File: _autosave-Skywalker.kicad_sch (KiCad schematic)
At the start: 28 parts

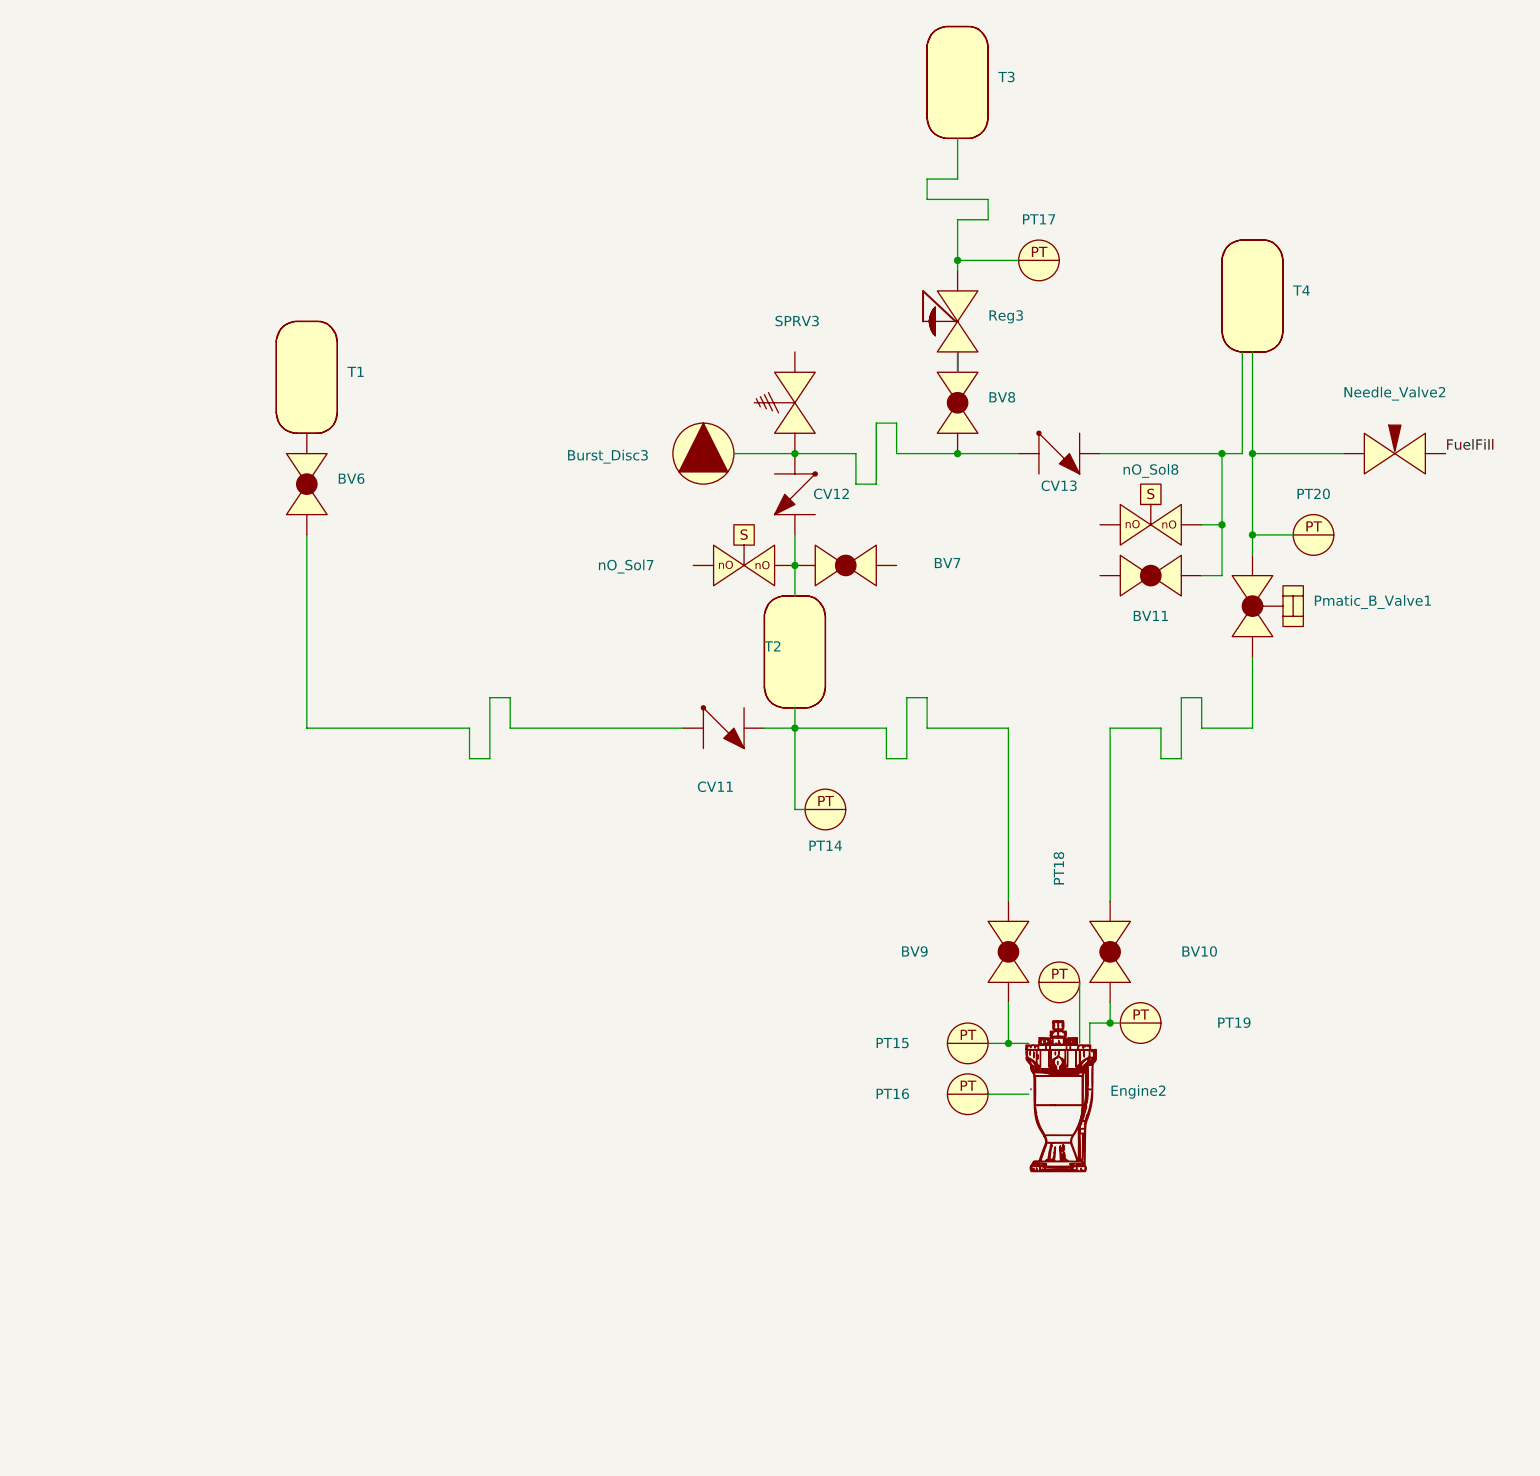
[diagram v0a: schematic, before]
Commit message: update
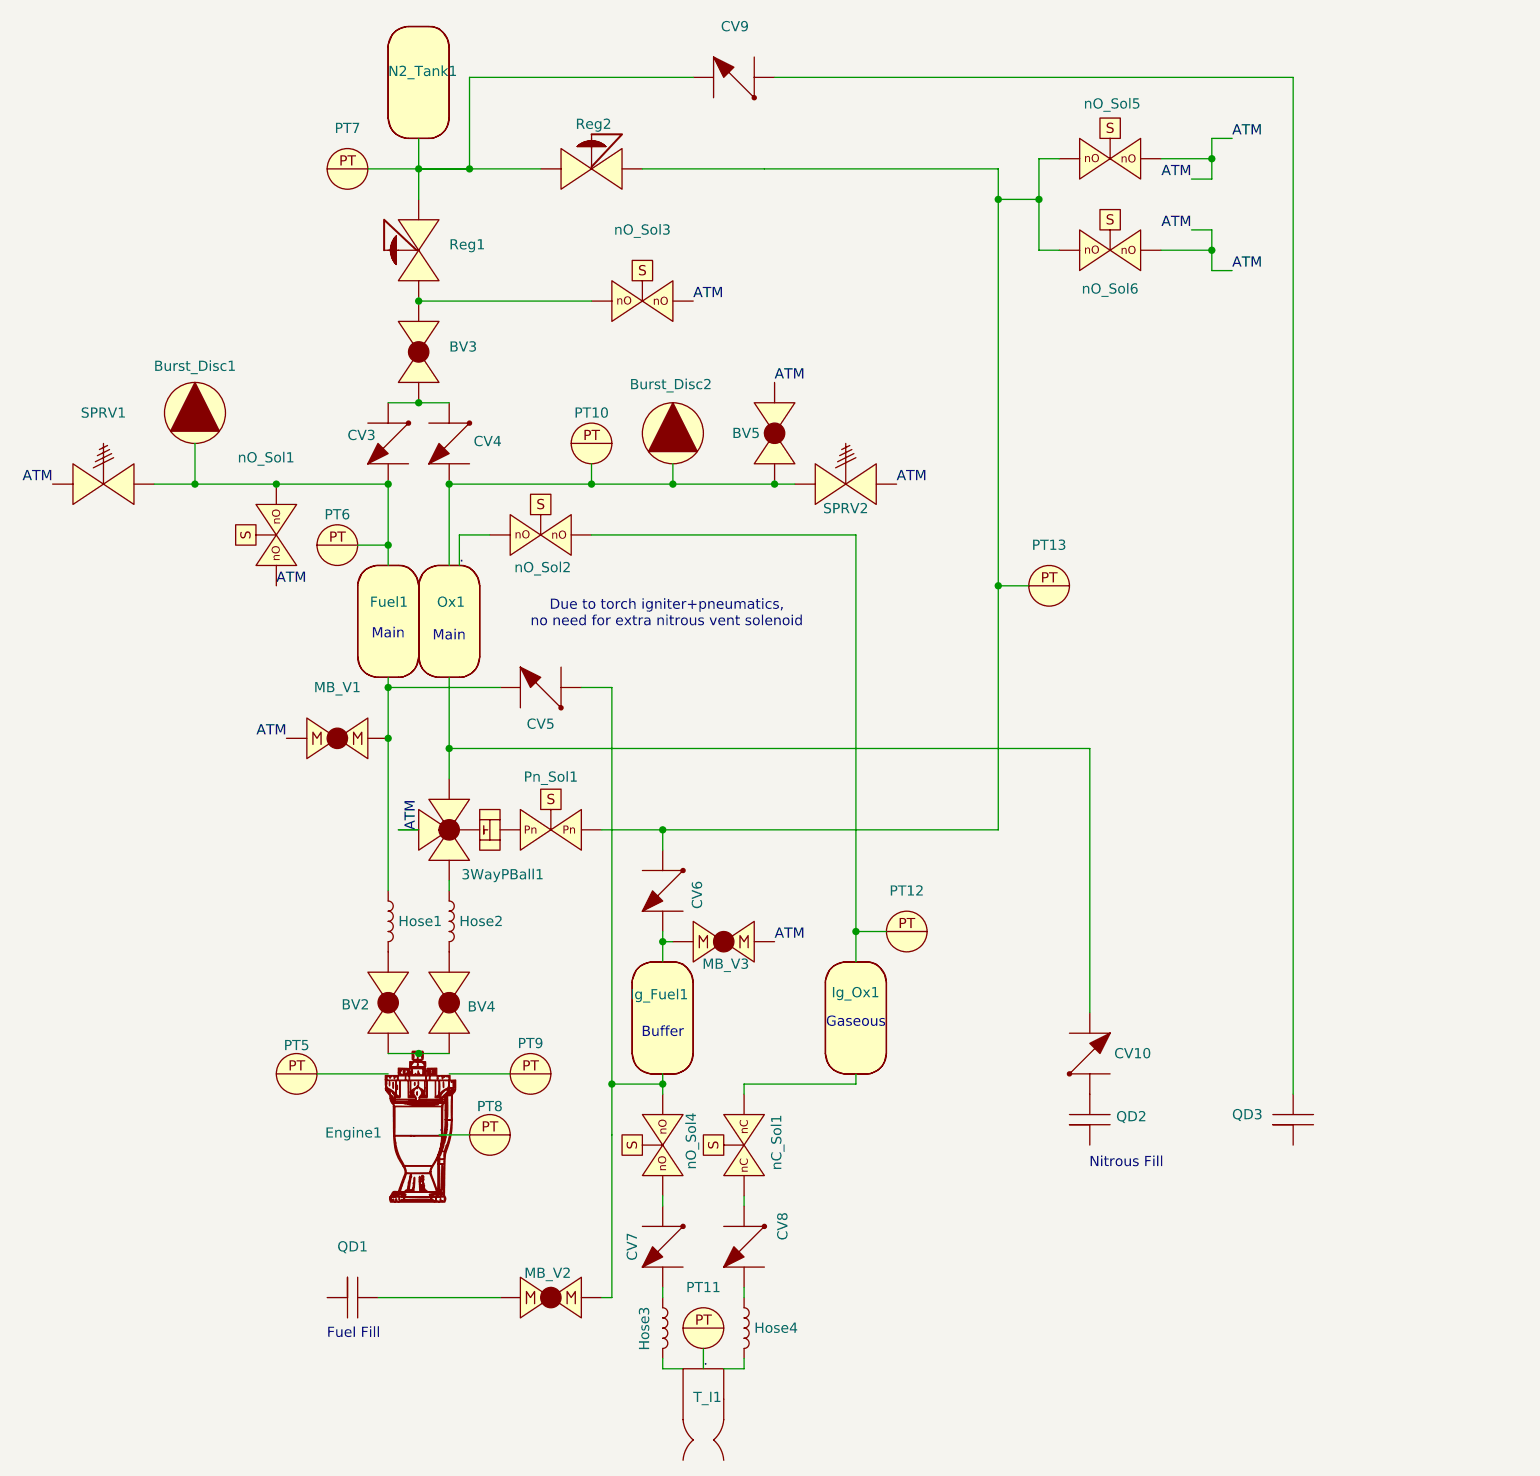
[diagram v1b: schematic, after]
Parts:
- removed BV10, BV11, BV6, BV7, BV8, BV9: ~, symbol PID_symbols:Ball_Valve
- removed Burst_Disc3: ~, symbol PID_symbols:Burst_Disc
- removed CV11, CV12, CV13: ~, symbol PID_symbols:Check_Valve
- removed Engine2: ~, symbol PID_symbols:Engine
- removed Needle_Valve2: ~, symbol PID_symbols:Needle_Valve
- removed PT14, PT15, PT16, PT17, PT18, PT19, PT20: ~, symbol PID_symbols:Pressure_Transducer
- removed Pmatic_B_Valve1: ~, symbol PID_symbols:Pneumatic_Rotary_Ball_Valve
- removed Reg3: ~, symbol PID_symbols:Pressure_Regulator
- removed SPRV3: ~, symbol PID_symbols:SPRV
- removed T1, T2, T3, T4: ~, symbol PID_symbols:Tank
- removed nO_Sol7, nO_Sol8: ~, symbol PID_symbols:Solenoid
- added 3WayPBall1: ~, symbol PID_symbols:3WayPmaticBall
- added BV2, BV3, BV4, BV5: ~, symbol PID_symbols:Ball_Valve
- added Burst_Disc1, Burst_Disc2: ~, symbol PID_symbols:Burst_Disc
- added CV10, CV3, CV4, CV5, CV6, CV7, CV8, CV9: ~, symbol PID_symbols:Check_Valve
- added Engine1: ~, symbol PID_symbols:Engine
- added Fuel1, Ig_Fuel1, Ig_Ox1, N2_Tank1, Ox1: ~, symbol PID_symbols:Tank
- added Hose1, Hose2, Hose3, Hose4: ~, symbol Device:Hose
- added MB_V1, MB_V2, MB_V3: ~, symbol PID_symbols:MBallValve
- added PT10, PT11, PT12, PT13, PT5, PT6, PT7, PT8, PT9: ~, symbol PID_symbols:Pressure_Transducer
- added Pn_Sol1: ~, symbol PID_symbols:Pneumatic_Solenoid
- added QD1, QD2, QD3: ~, symbol PID_symbols:Quick_Disconnect
- added Reg1, Reg2: ~, symbol PID_symbols:Pressure_Regulator
- added SPRV1, SPRV2: ~, symbol PID_symbols:SPRV
- added T_I1: ~, symbol Analog_ADC:Torch_Igniter
- added nC_Sol1: ~, symbol PID_symbols:Normally_Closed_Solenoid
- added nO_Sol1, nO_Sol2, nO_Sol3, nO_Sol4, nO_Sol5, nO_Sol6: ~, symbol PID_symbols:Solenoid
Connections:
- net .: now also PT11., PT8., nO_Sol2.
- new net: CV9., N2_Tank1., PT7., Reg1., Reg2.
- new net: CV6., PT13., Pn_Sol1., Reg2., nO_Sol5., nO_Sol6.
- new net: CV6., Ig_Fuel1., MB_V3.
- new net: Engine1., PT9.
- new net: BV2., BV4., Engine1.
- new net: Engine1., PT5.
- new net: CV9., QD3.
- new net: CV5., Ig_Fuel1., MB_V2., nO_Sol4.
- new net: MB_V2., QD1.
- new net: BV4., Hose2.2
- new net: CV8., nC_Sol1.
- new net: CV8., Hose4.1
- new net: Burst_Disc1., CV3., Fuel1., PT6., SPRV1., nO_Sol1.
- new net: BV3., CV3., CV4.
- new net: CV5., Fuel1., Hose1.1, MB_V1.
- new net: BV2., Hose1.2
- new net: CV7., Hose3.1
- new net: Hose3.2, T_I1.
- new net: Ig_Ox1., PT12., nO_Sol2.
- new net: Ig_Ox1., nC_Sol1.
- new net: CV7., nO_Sol4.
- new net: 3WayPBall1., Pn_Sol1.
- new net: 3WayPBall1., CV10., Ox1.
- new net: 3WayPBall1., Hose2.1
- new net: BV5., Burst_Disc2., CV4., Ox1., PT10., SPRV2.
- new net: CV10., QD2.
- new net: BV3., Reg1., nO_Sol3.
- new net: Hose4.2, T_I1.
- new net ATM: 3WayPBall1., BV5., MB_V1., MB_V3., SPRV1., SPRV2., nO_Sol1., nO_Sol3., nO_Sol5., nO_Sol6.
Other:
- note added: "Buffer"
- note added: "Due to torch igniter+pneumatics, no need for extra nitrous vent solenoid"
- note added: "Fuel Fill"
- note added: "Gaseous"
- note added: "Main"
- note added: "Nitrous Fill"
